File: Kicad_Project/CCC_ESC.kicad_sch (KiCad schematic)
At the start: 225 parts, among them J1 Conn_01x07, J2 Conn_01x06, J3 Conn_01x06, J4 Conn_01x06, SW1 Conn_01x02, U1 NCP5183 / TF2190-TAH, U2 NCP5183 / TF2190-TAH, U3 NCP5183 / TF2190-TAH, U4 NCS20034DR2G, U5 STM32F401CCU6_Balckpill, U6 PQDE6W-Q110 / RD5-110S12W, U7 TO220_replacement_module

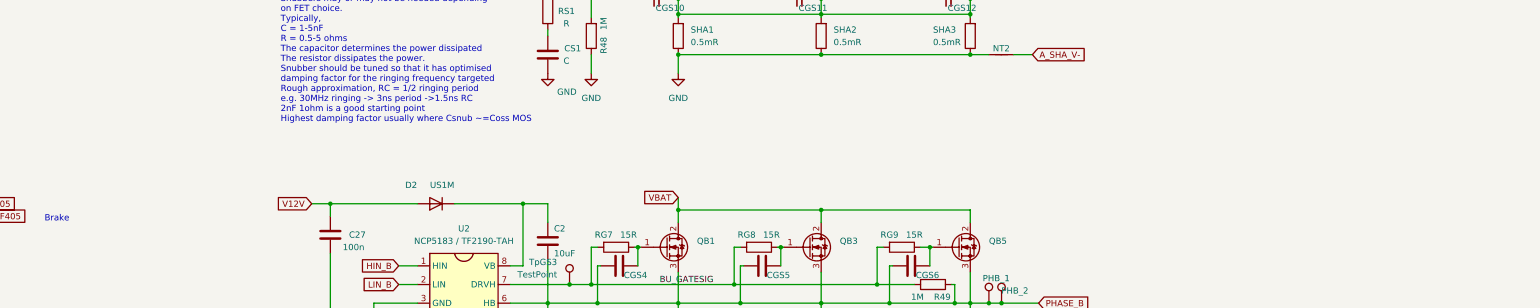
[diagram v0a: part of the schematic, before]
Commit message: first draft
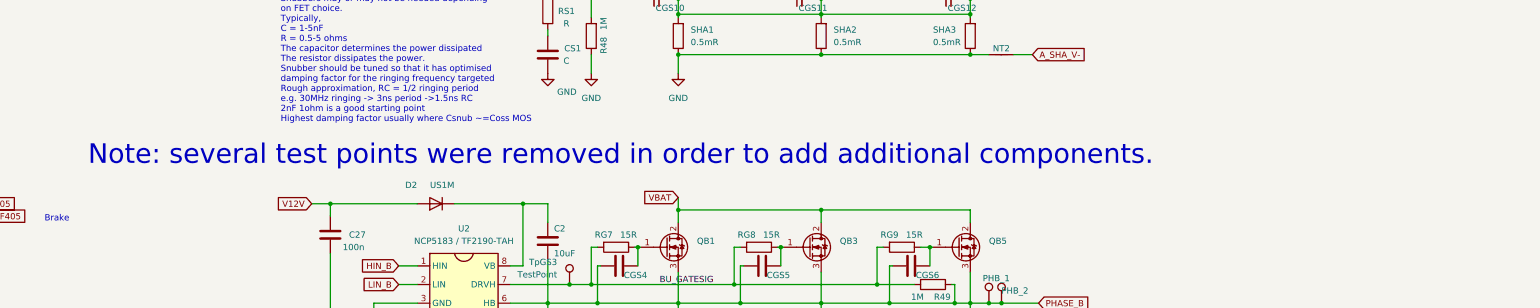
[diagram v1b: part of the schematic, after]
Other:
- note added: "Note: several test points were removed in order to add additional components."
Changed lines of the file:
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@@
     (effects (font (size 1.27 1.27)) (justify left bottom))
+  )
+  (text "Note: several test points were removed in order to add additional components."
+    (at 354.33 132.08 0)
+    (effects (font (size 4 4)) (justify left bottom))
   )
   (text "Phase sensing" (at 312.42 154.94 0)
